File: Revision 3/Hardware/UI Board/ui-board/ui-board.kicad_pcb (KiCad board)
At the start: 6 copper layers, 109 x 75 mm, 13 parts, among them J1 Conn_01x07, SW1 SW_Push_45deg, SW10 SW_Push_45deg, SW11 SW_Push_45deg, SW12 SW_Push_45deg, SW2 SW_Push_45deg, SW3 SW_Push_45deg, SW4 SW_Push_45deg, SW5 SW_Push_45deg, SW6 SW_Push_45deg, SW7 SW_Push_45deg, SW8 SW_Push_45deg, SW9 SW_Push_45deg

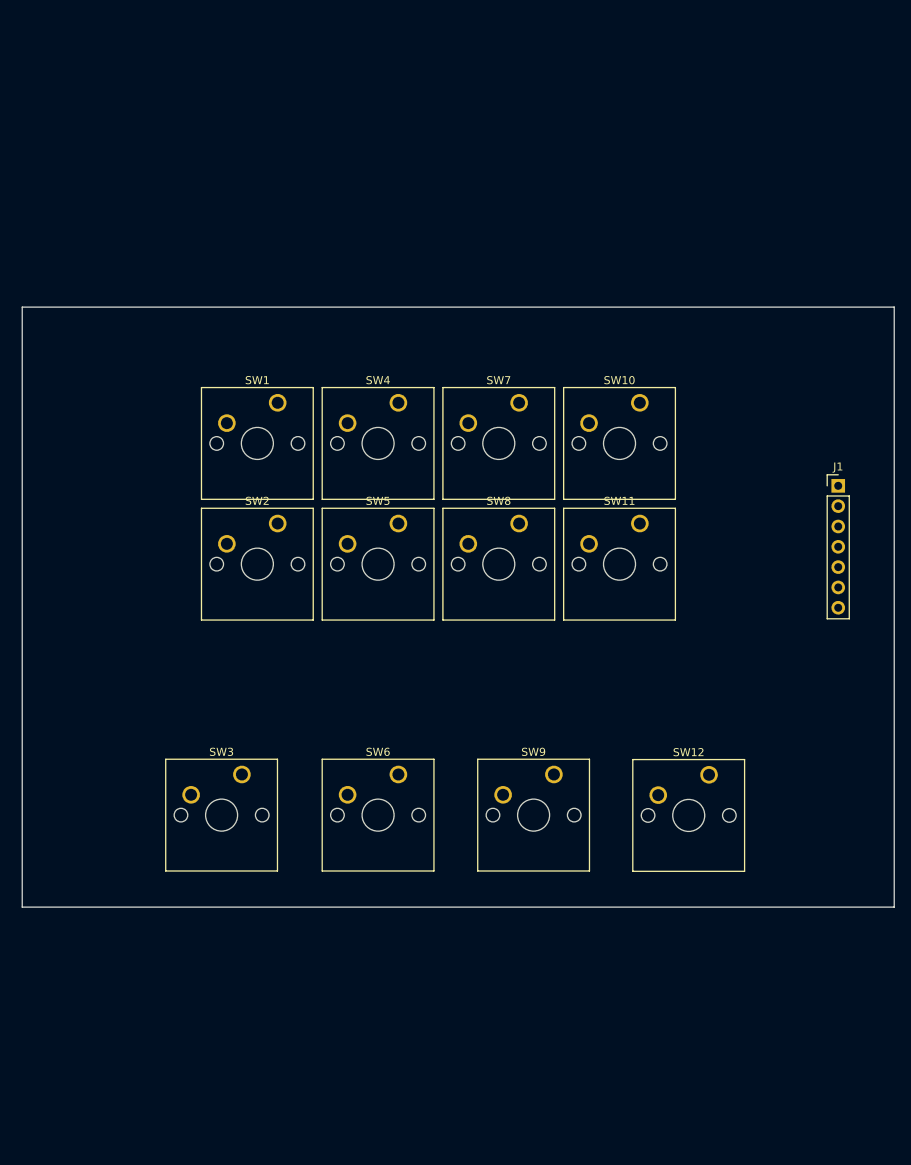
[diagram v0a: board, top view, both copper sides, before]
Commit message: board complete and fab files generated, sent to fab
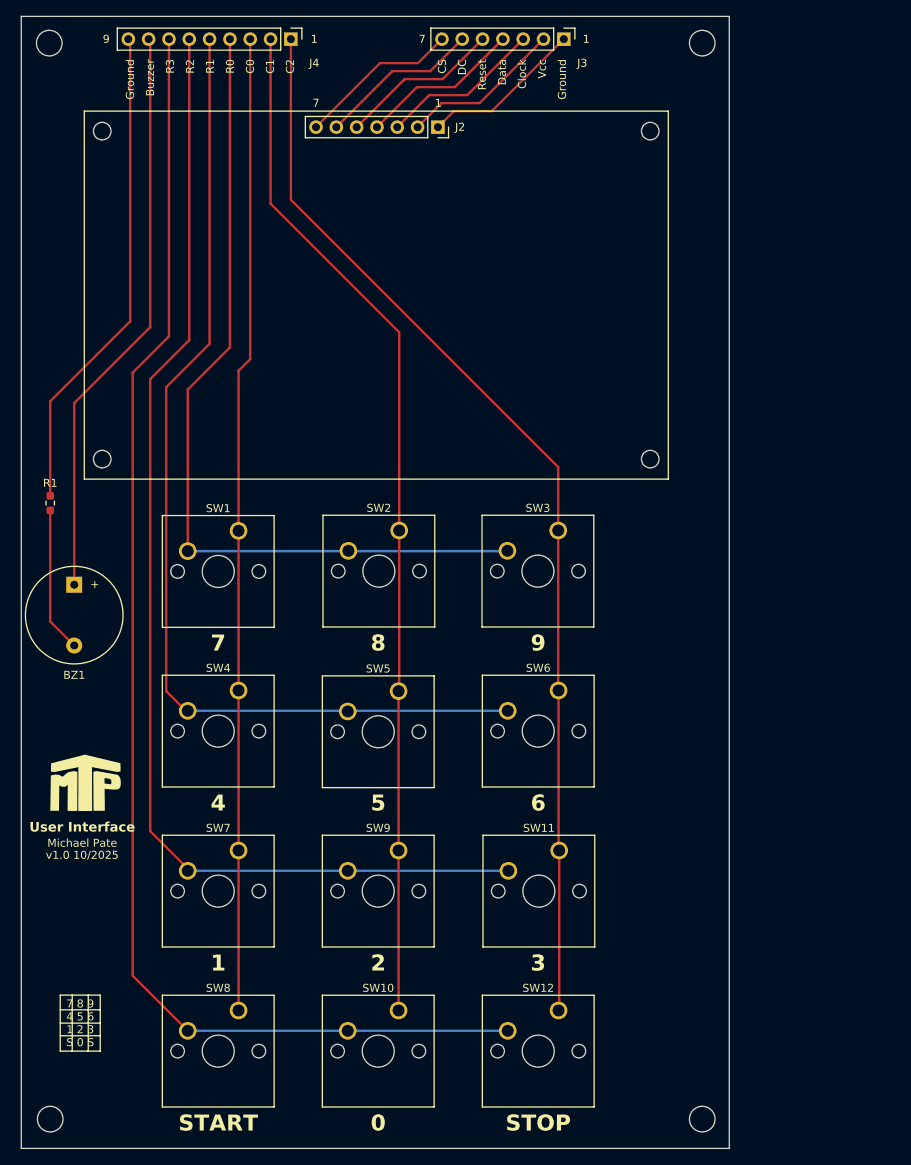
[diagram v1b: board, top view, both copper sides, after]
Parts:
- removed J1: Conn_01x07, Connector_PinHeader_2.54mm:PinHeader_1x07_P2.54mm_Vertical
- added BZ1: PT-1306T, Buzzer_Beeper:Buzzer_12x9.5RM7.6, F.Cu at (120.0, 84.7)
- added H1: MountingHole, MountingHole:MountingHole_3.2mm_M3, F.Cu at (116.9, 17.0)
- added H2: MountingHole, MountingHole:MountingHole_3.2mm_M3, F.Cu at (117.0, 151.5)
- added H3: MountingHole, MountingHole:MountingHole_3.2mm_M3, F.Cu at (198.5, 17.0)
- added H4: MountingHole, MountingHole:MountingHole_3.2mm_M3, F.Cu at (198.5, 151.5)
- added H5: MountingHole, MountingHole:MountingHole_2.2mm_M2, F.Cu at (123.5, 28.0)
- added H6: MountingHole, MountingHole:MountingHole_2.2mm_M2, F.Cu at (192.0, 28.0)
- added H7: MountingHole, MountingHole:MountingHole_2.2mm_M2, F.Cu at (123.5, 69.0)
- added H8: MountingHole, MountingHole:MountingHole_2.2mm_M2, F.Cu at (192.0, 69.0)
- added J2: Conn_01x07, Connector_PinSocket_2.54mm:PinSocket_1x07_P2.54mm_Vertical, F.Cu at (165.5, 27.5)
- added J3: Conn_01x07, Connector_PinHeader_2.54mm:PinHeader_1x07_P2.54mm_Vertical, F.Cu at (181.2, 16.5)
- added J4: Conn_01x09, Connector_PinHeader_2.54mm:PinHeader_1x09_P2.54mm_Vertical, F.Cu at (147.1, 16.5)
- added R1: 1k, Resistor_SMD:R_0603_1608Metric_Pad0.98x0.95mm_HandSolder, F.Cu at (117.0, 74.5)
- added REF**: MTP Logo 10mm Low Detail, Watermarks:MTP Logo 10mm Low Detail, F.Cu at (121.5, 109.5)
- moved SW10 81.7 mm to (160.5, 137.9)
- moved SW8 70.2 mm to (140.5, 137.9)
- moved SW7 66.0 mm to (140.5, 117.9)
- moved SW3 49.9 mm to (180.5, 77.9)
- moved SW11 42.1 mm to (180.6, 117.9)
- moved SW4 41.1 mm to (140.5, 97.9)
- moved SW12 35.0 mm to (180.5, 137.9)
- moved SW6 22.6 mm to (180.5, 97.9)
- moved SW9 21.6 mm to (160.5, 117.9)
- moved SW5 21.0 mm to (160.5, 98.0)
- moved SW1 16.7 mm to (140.5, 78.0)
- moved SW2 15.2 mm to (160.6, 77.9)
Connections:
- net Net-(J1-Pin_1) renamed /User Interface/Col_0
- net Net-(J1-Pin_2) renamed /User Interface/Col_1
- net Net-(J1-Pin_3) renamed /User Interface/Col_2
- net Net-(J1-Pin_4) renamed /User Interface/Row_0
- net Net-(J1-Pin_5) renamed /User Interface/Row_1
- net Net-(J1-Pin_6) renamed /User Interface/Row_2
- net Net-(J1-Pin_7) renamed /User Interface/Row_3
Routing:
- net /User Interface/Row_3: track 0.00 -> 168.7 mm
- net /User Interface/Row_2: track 0.00 -> 148.0 mm
- net /User Interface/Col_2: track 0.00 -> 135.3 mm
- net /User Interface/Col_1: track 0.00 -> 128.1 mm
- net /User Interface/Row_1: track 0.00 -> 127.5 mm
- net /User Interface/Col_0: track 0.00 -> 122.0 mm
- net /User Interface/Row_0: track 0.00 -> 106.2 mm
- net Net-(BZ1-+): track 0.00 -> 72.2 mm
- net Net-(J4-Pin_9): track 0.00 -> 61.3 mm
- net /User Interface/LCD_VCC: track 0.00 -> 20.3 mm
- net /User Interface/LCD_SDA: track 0.00 -> 20.3 mm
- net /User Interface/LCD_CS: track 0.00 -> 20.3 mm
- net /User Interface/LCD_SCK: track 0.00 -> 20.3 mm
- net /User Interface/LCD_DC: track 0.00 -> 20.3 mm
- net /User Interface/LCD_RES: track 0.00 -> 20.3 mm
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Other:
- board size 109 x 75 mm -> 88.5 x 141.5 mm
- board text added: "0"
- board text added: "1"
- board text added: "2"
- board text added: "3"
- board text added: "4"
- board text added: "5"
- board text added: "6"
- board text added: "7"
- board text added: "7 8 9 4 5 6 1 2 3 S 0 S"
- board text added: "8"
- board text added: "9"
- board text added: "Buzzer"
- board text added: "C0"
- board text added: "C1"
- board text added: "C2"
- board text added: "CS"
- board text added: "Clock"
- board text added: "DC"
- board text added: "Data"
- board text added: "Ground"
- board text added: "Michael Pate"
- board text added: "R0"
- board text added: "R1"
- board text added: "R2"
- board text added: "R3"
- board text added: "Reset"
- board text added: "START"
- board text added: "STOP"
- board text added: "User Interface"
- board text added: "Vcc"
- board text added: "v1.0 10/2025"
